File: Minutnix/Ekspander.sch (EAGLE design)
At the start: 14 parts, among them X1 FH12-12S-0.5S_THINNER, X6 JST-XH-03-PIN-LONG-PAD

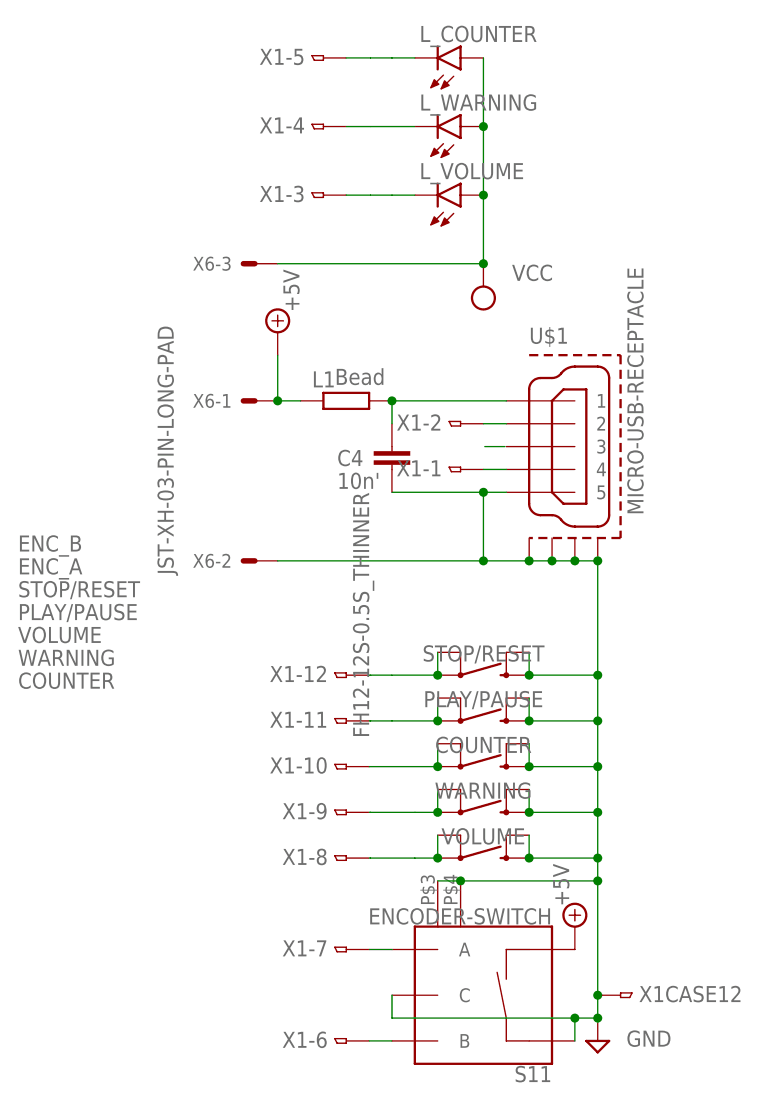
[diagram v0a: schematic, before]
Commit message: Many final changes
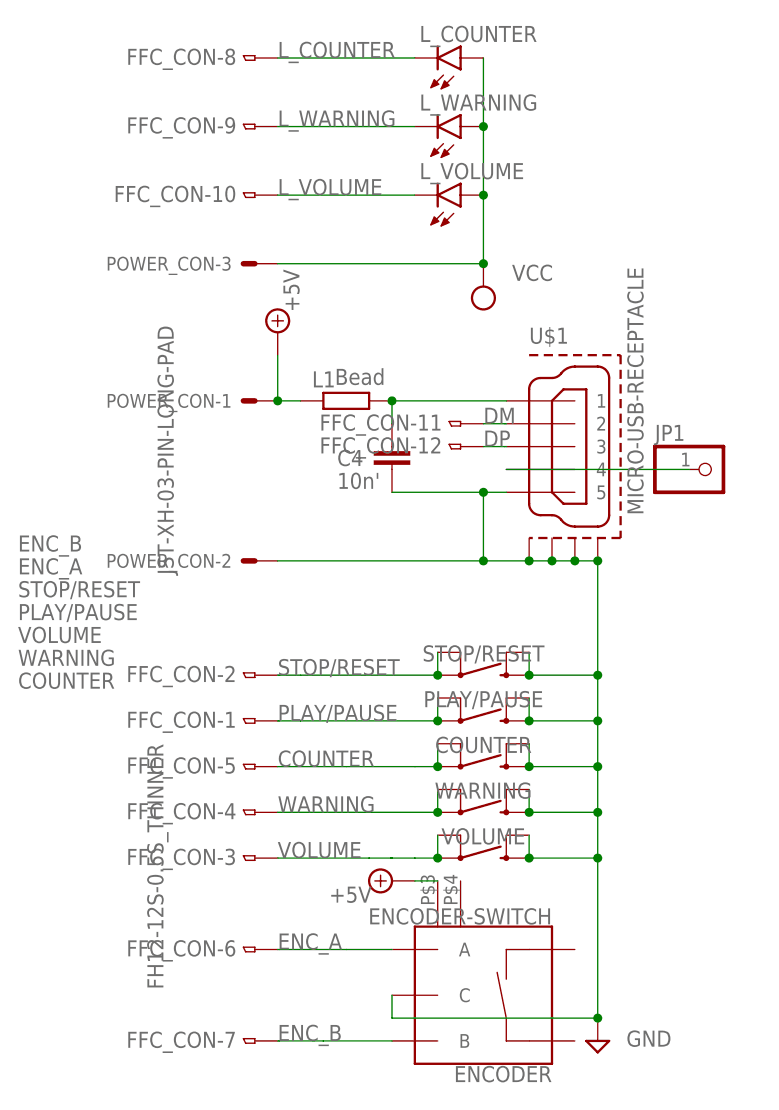
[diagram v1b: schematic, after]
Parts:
- removed X1: FH12-12S-0.5S_THINNER, My_con-hirose:FH12-12S-0.5S_THINNER
- added FFC_CON: FH12-12S-0.5S_THINNER, My_con-hirose:FH12-12S-0.5S_THINNER
- added JP1: (no value), pinhead:PINHD-1X1
- renumbered S11 to ENCODER, X6 to POWER_CON
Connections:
- removed net N$1: ENCODER.A, X1-7.1
- removed net N$10: L_COUNTER.C, X1-5.1
- removed net N$11: L_WARNING.C, X1-4.1
- removed net N$12: L_VOLUME.C, X1-3.1
- removed net N$17: U$1.4, X1-1.1
- removed net N$18: U$1.2, X1-2.1
- removed net N$2: STOP/RESET.1, STOP/RESET.3, X1-12.1
- removed net N$3: PLAY/PAUSE.1, PLAY/PAUSE.3, X1-11.1
- removed net N$4: COUNTER.1, COUNTER.3, X1-10.1
- removed net N$5: WARNING.1, WARNING.3, X1-9.1
- removed net N$6: VOLUME.1, VOLUME.3, X1-8.1
- removed net N$7: ENCODER.B, X1-6.1
- new net COUNTER: COUNTER.1, COUNTER.3, FFC_CON-5.1
- new net DM: FFC_CON-11.1, U$1.2
- new net DP: FFC_CON-12.1, U$1.3
- new net ENC_A: ENCODER.A, FFC_CON-6.1
- new net ENC_B: ENCODER.B, FFC_CON-7.1
- new net L_COUNTER: FFC_CON-8.1, L_COUNTER.C
- new net L_VOLUME: FFC_CON-10.1, L_VOLUME.C
- new net L_WARNING: FFC_CON-9.1, L_WARNING.C
- new net N$8: JP1.1, U$1.4
- new net PLAY/PAUSE: FFC_CON-1.1, PLAY/PAUSE.1, PLAY/PAUSE.3
- new net STOP/RESET: FFC_CON-2.1, STOP/RESET.1, STOP/RESET.3
- new net VOLUME: FFC_CON-3.1, VOLUME.1, VOLUME.3
- new net WARNING: FFC_CON-4.1, WARNING.1, WARNING.3
- net +5V: now also ENCODER.GND1; no longer ENCODER.SW-
- net GND: no longer ENCODER.GND1, ENCODER.GND2, ENCODER.SW+, X1CASE12.1
